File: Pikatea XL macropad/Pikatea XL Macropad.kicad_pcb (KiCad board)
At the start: 2 copper layers, 118.6 x 37.2 mm, 11 parts, among them J1 Conn_01x12_Female, SW3 Rotary_Encoder_Switch, U1 ProMicro

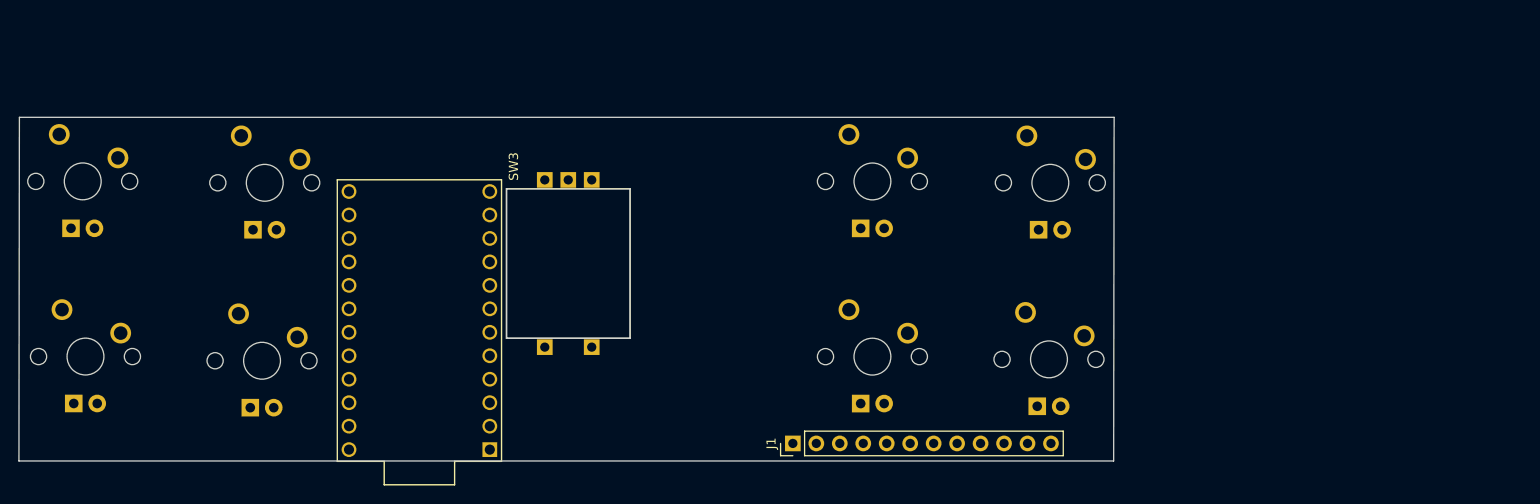
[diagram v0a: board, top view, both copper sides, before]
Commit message: updates to XL macropad
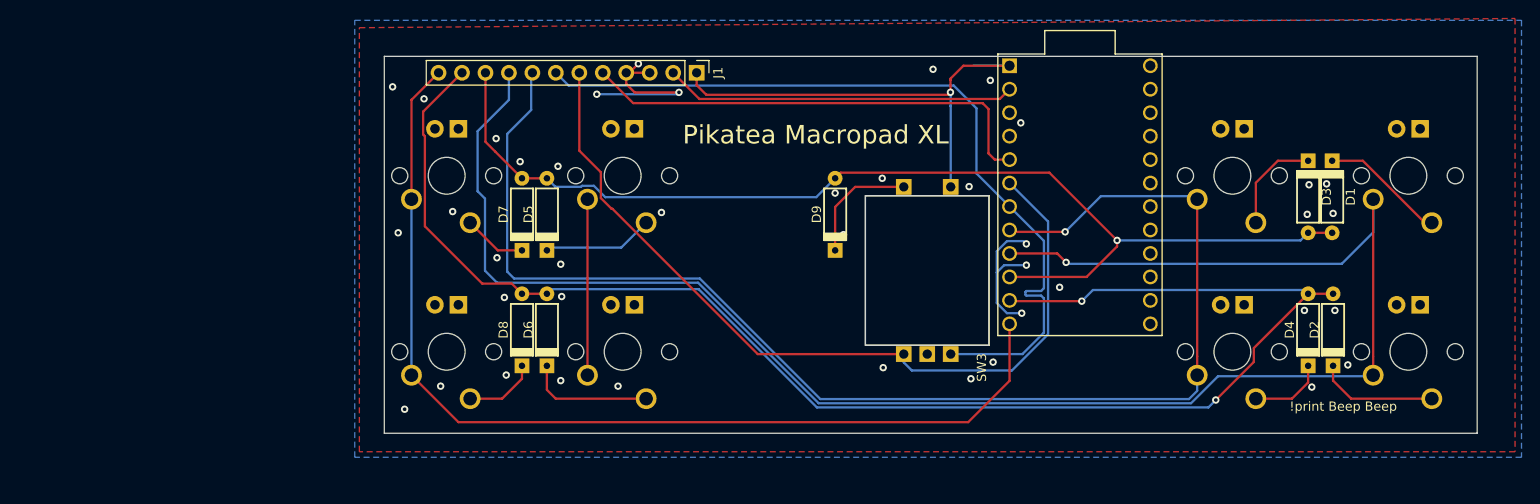
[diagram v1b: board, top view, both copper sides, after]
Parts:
- added D1: 1N4148W, keyboard_parts:D_axial, F.Cu at (190.9, 90.6)
- added D2: 1N4148W, keyboard_parts:D_axial, F.Cu at (191.0, 105.0)
- added D3: 1N4148W, keyboard_parts:D_axial, F.Cu at (188.3, 90.6)
- added D4: 1N4148W, keyboard_parts:D_axial, F.Cu at (188.3, 105.0)
- added D5: 1N4148W, keyboard_parts:D_axial, F.Cu at (105.9, 92.5)
- added D6: 1N4148W, keyboard_parts:D_axial, F.Cu at (105.9, 105.0)
- added D7: 1N4148W, keyboard_parts:D_axial, F.Cu at (103.2, 92.5)
- added D8: 1N4148W, keyboard_parts:D_axial, F.Cu at (103.2, 105.0)
- added D9: 1N4148W, keyboard_parts:D_axial, F.Cu at (137.1, 92.5)
- moved MX1 144.7 mm to (199.2, 107.4), turned to 0 degrees
- moved MX5 144.5 mm to (199.2, 88.3), turned to 0 degrees
- moved MX6 106.9 mm to (180.1, 88.3), turned to 0 degrees
- moved MX2 106.3 mm to (180.1, 107.4), turned to 0 degrees
- moved U1 72.8 mm to (163.6, 90.4), turned to 270 degrees
- moved MX8 68.2 mm to (95.1, 88.3), turned to 0 degrees
- moved MX4 67.9 mm to (95.1, 107.4), turned to 0 degrees
- moved J1 41.5 mm to (122.1, 77.2), turned to 270 degrees
- moved SW3 38.9 mm to (147.1, 98.6), turned to 90 degrees
- moved MX7 33.4 mm to (114.1, 88.3), turned to 0 degrees
- moved MX3 32.7 mm to (114.1, 107.4), turned to 0 degrees
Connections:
- J1 pad 1: (no net) -> /A10
- J1 pad 10: (no net) -> /A3
- J1 pad 11: (no net) -> /A0
- J1 pad 12: (no net) -> /A4
- J1 pad 2: (no net) -> Net-(J1-Pad2)
- J1 pad 3: (no net) -> GND
- J1 pad 4: (no net) -> GND
- J1 pad 5: (no net) -> Net-(J1-Pad5)
- J1 pad 6: (no net) -> /B
- J1 pad 7: (no net) -> /A
- J1 pad 8: (no net) -> /D7
- J1 pad 9: (no net) -> /D9
- MX1 pad 3: (no net) -> Net-(MX1-Pad3)
- MX1 pad 4: (no net) -> Net-(MX1-Pad4)
- MX2 pad 3: (no net) -> Net-(MX2-Pad3)
- MX2 pad 4: (no net) -> Net-(MX2-Pad4)
- MX3 pad 3: (no net) -> Net-(MX3-Pad3)
- MX3 pad 4: (no net) -> Net-(MX3-Pad4)
- MX4 pad 3: (no net) -> Net-(MX4-Pad3)
- MX4 pad 4: (no net) -> Net-(MX4-Pad4)
- MX5 pad 3: (no net) -> Net-(MX5-Pad3)
- MX5 pad 4: (no net) -> Net-(MX5-Pad4)
- MX6 pad 3: (no net) -> Net-(MX6-Pad3)
- MX6 pad 4: (no net) -> Net-(MX6-Pad4)
- MX7 pad 3: (no net) -> Net-(MX7-Pad3)
- MX7 pad 4: (no net) -> Net-(MX7-Pad4)
- MX8 pad 3: (no net) -> Net-(MX8-Pad3)
- MX8 pad 4: (no net) -> Net-(MX8-Pad4)
- SW3 pad A: (no net) -> /A
- SW3 pad B: (no net) -> /B
- SW3 pad C: (no net) -> GND
- SW3 pad S2: (no net) -> /A10
- U1 pad 1: (no net) -> /A10
- U1 pad 10: (no net) -> /A3
- U1 pad 11: (no net) -> /A0
- U1 pad 12: (no net) -> /A4
- U1 pad 13: (no net) -> Net-(U1-Pad13)
- U1 pad 14: (no net) -> Net-(U1-Pad14)
- U1 pad 15: (no net) -> Net-(U1-Pad15)
- U1 pad 16: (no net) -> Net-(U1-Pad16)
- U1 pad 17: (no net) -> Net-(U1-Pad17)
- U1 pad 18: (no net) -> Net-(U1-Pad18)
- U1 pad 19: (no net) -> Net-(U1-Pad19)
- U1 pad 2: (no net) -> Net-(J1-Pad2)
- U1 pad 20: (no net) -> Net-(U1-Pad20)
- U1 pad 21: (no net) -> Net-(U1-Pad21)
- U1 pad 22: (no net) -> Net-(U1-Pad22)
- U1 pad 23: (no net) -> Net-(U1-Pad23)
- U1 pad 24: (no net) -> Net-(U1-Pad24)
- U1 pad 3: (no net) -> GND
- U1 pad 4: (no net) -> GND
- U1 pad 5: (no net) -> Net-(J1-Pad5)
- U1 pad 6: (no net) -> /B
- U1 pad 7: (no net) -> /A
- U1 pad 8: (no net) -> /D7
- U1 pad 9: (no net) -> /D9
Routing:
- net /D9: track 0.00 -> 190.4 mm, vias 0 -> 1
- net /A0: track 0.00 -> 164.3 mm, vias 0 -> 2
- net /D7: track 0.00 -> 146.3 mm, vias 0 -> 1
- net /A3: track 0.00 -> 120.7 mm, vias 0 -> 1
- net /A4: track 0.00 -> 108.8 mm
- net /B: track 0.00 -> 90.9 mm
- net /A: track 0.00 -> 89.0 mm
- net /A10: track 0.00 -> 52.1 mm, vias 0 -> 1
- net Net-(J1-Pad5): track 0.00 -> 50.9 mm
- net Net-(J1-Pad2): track 0.00 -> 38.0 mm
- net GND: track 0.00 -> 36.6 mm, vias 0 -> 42
- net /D8: track 0.00 -> 19.0 mm
- net Net-(D6-Pad1): track 0.00 -> 13.7 mm
- net Net-(D1-Pad1): track 0.00 -> 13.6 mm
- net Net-(D2-Pad1): track 0.00 -> 13.1 mm
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- added copper zone on B.Cu, net GND
- added copper zone on F.Cu, net GND
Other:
- board size 118.6 x 37.2 mm -> 118.3 x 40.8 mm
- board text added: "!print Beep Beep"
- board text added: "Pikatea Macropad XL"
